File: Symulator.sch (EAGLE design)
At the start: 10 parts

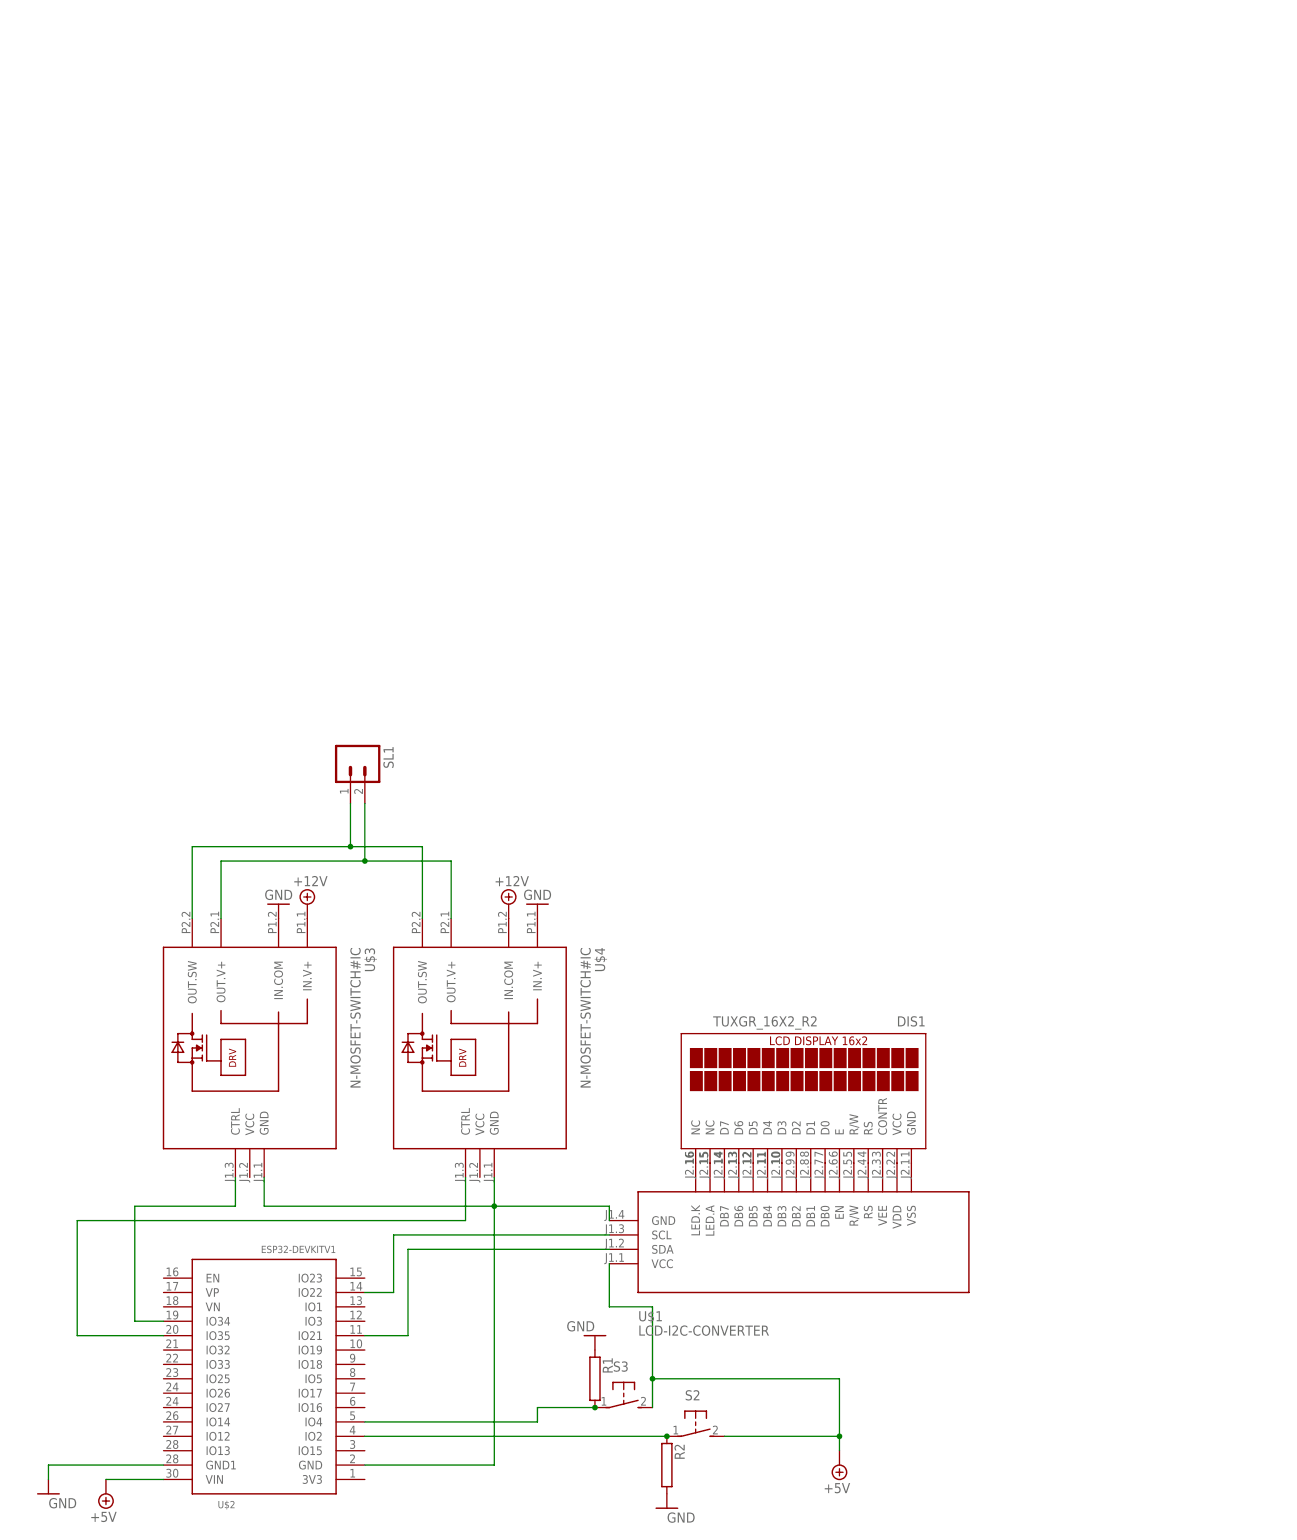
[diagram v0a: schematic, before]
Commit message: Add files via upload
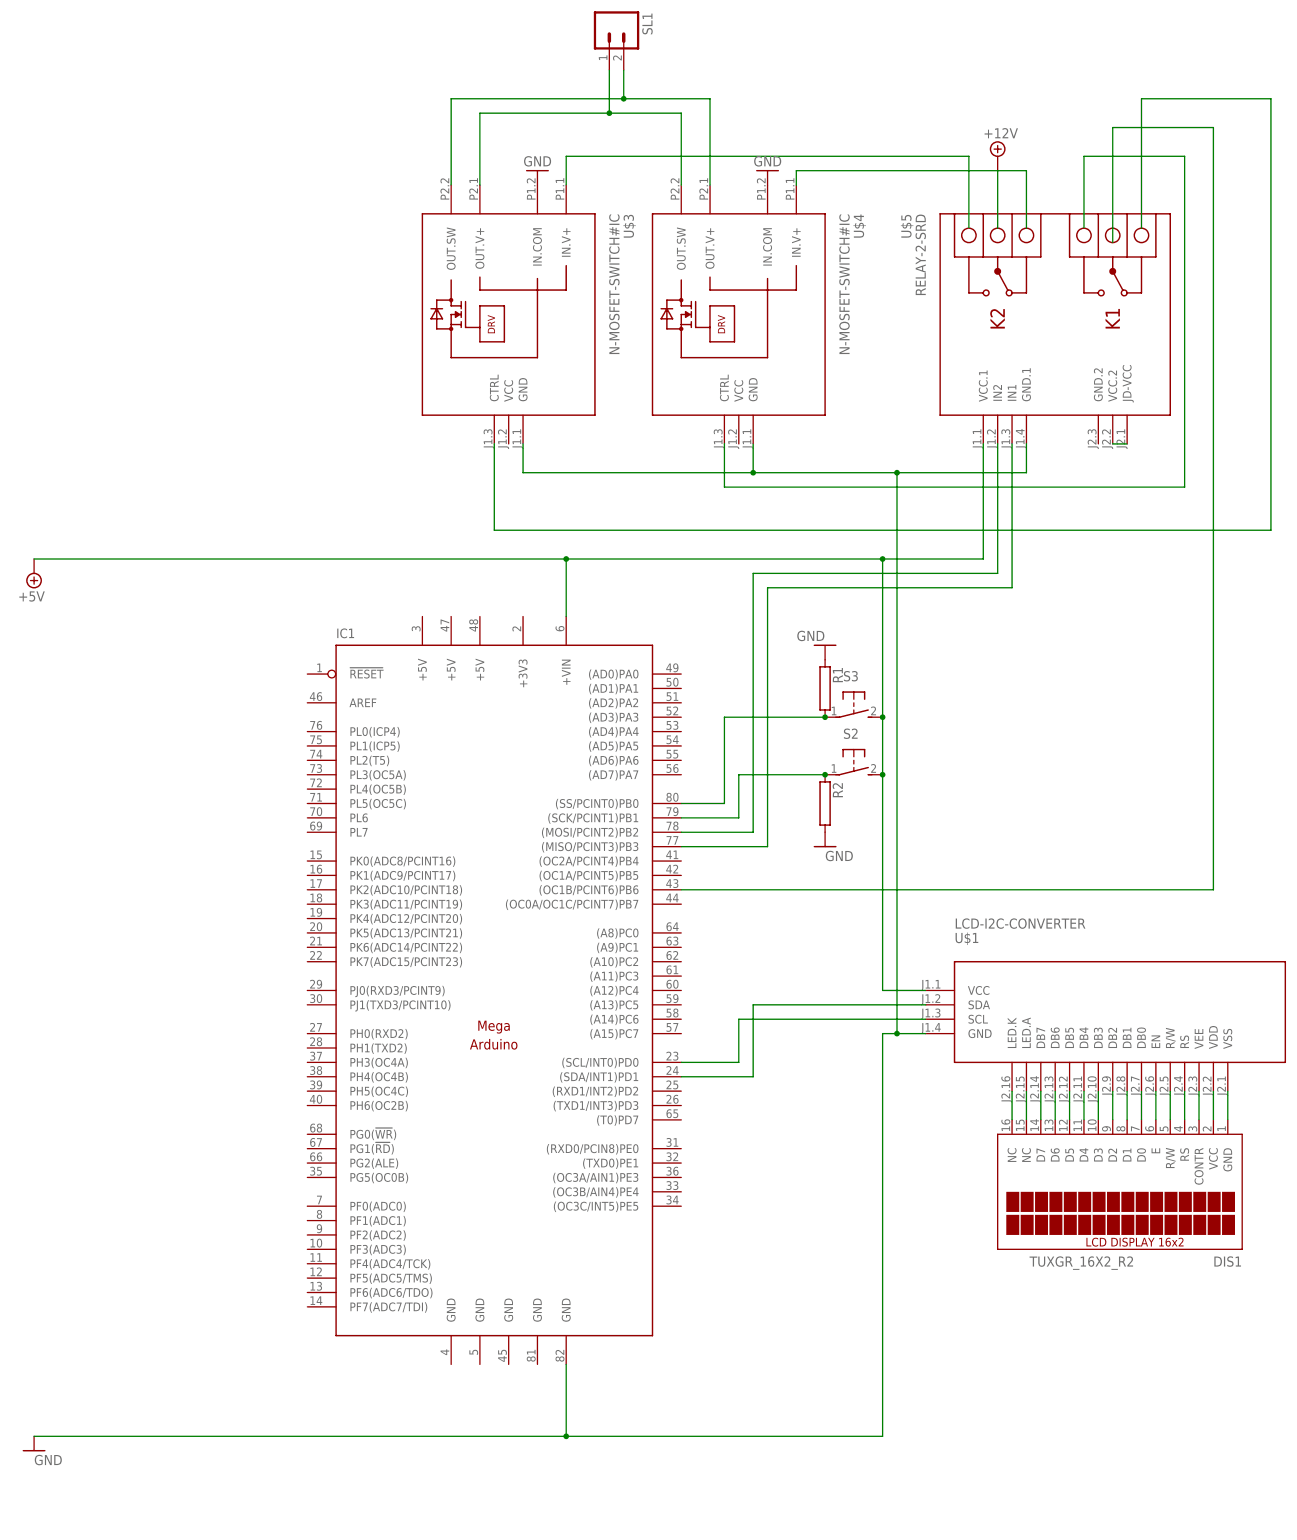
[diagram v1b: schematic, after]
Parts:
- removed U$2: ESP32DEVKITV1, ESP32-DEVKITV1:ESP32DEVKITV1
- added IC1: (no value), arduino:MEGAARDUINO_11
- added U$5: RELAY-2-SRD, diy-modules:RELAY-2-SRD
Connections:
- removed net +12V: U$3.IN.V+, U$4.IN.COM
- removed net N$23: U$1.SDA, U$2.IO21
- new net N$26: SL1.2, U$3.OUT.SW, U$4.OUT.V+
- new net N$27: U$3.CTRL
- new net N$28: U$4.IN.V+
- new net N$29: U$3.IN.V+
- new net N$30: U$4.CTRL
- new net N$31: IC1.(MOSI/PCINT2)PB2, U$5.IN2
- net +5V: now also IC1.+VIN, U$5.VCC.1; no longer U$2.VIN
- net GND: now also IC1.GND@5, U$1.GND, U$3.GND, U$4.GND, U$4.IN.COM, U$5.GND.1; no longer U$2.GND1, U$4.IN.V+
- net N$17: now also IC1.(SCK/PCINT1)PB1; no longer U$2.IO2
- net N$18: now also SL1.1, U$3.OUT.V+, U$4.OUT.SW; no longer R1.2, S3.P, U$2.IO4
- net N$19: now also IC1.(SS/PCINT0)PB0, R1.2, S3.P; no longer U$2.IO34, U$3.CTRL
- net N$20: now also IC1.(SCL/INT0)PD0, U$1.SCL; no longer U$1.GND, U$2.GND, U$3.GND, U$4.GND
- net N$21: now also IC1.(SDA/INT1)PD1, U$1.SDA; no longer U$2.IO35, U$4.CTRL
- net N$22: now also IC1.(MISO/PCINT3)PB3, U$5.IN1; no longer U$1.SCL, U$2.IO22
- net N$24: now also U$5.JD-VCC, U$5.VCC.2; no longer SL1.1, U$3.OUT.SW, U$4.OUT.SW
- net N$25: now also IC1.(OC1B/PCINT6)PB6; no longer SL1.2, U$3.OUT.V+, U$4.OUT.V+
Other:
- moved on the sheet: DIS1, R1, R2, S2, S3, SL1, U$1, U$3, U$4
